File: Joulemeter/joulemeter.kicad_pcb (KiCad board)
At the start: 2 copper layers, 78.9 x 89.7 mm, 50 parts, among them J1 XT60-M, J2 XT60-M, J3 22035035, U2 MCP6286T-E/OT, U5 PADS131M04QPWRQ1

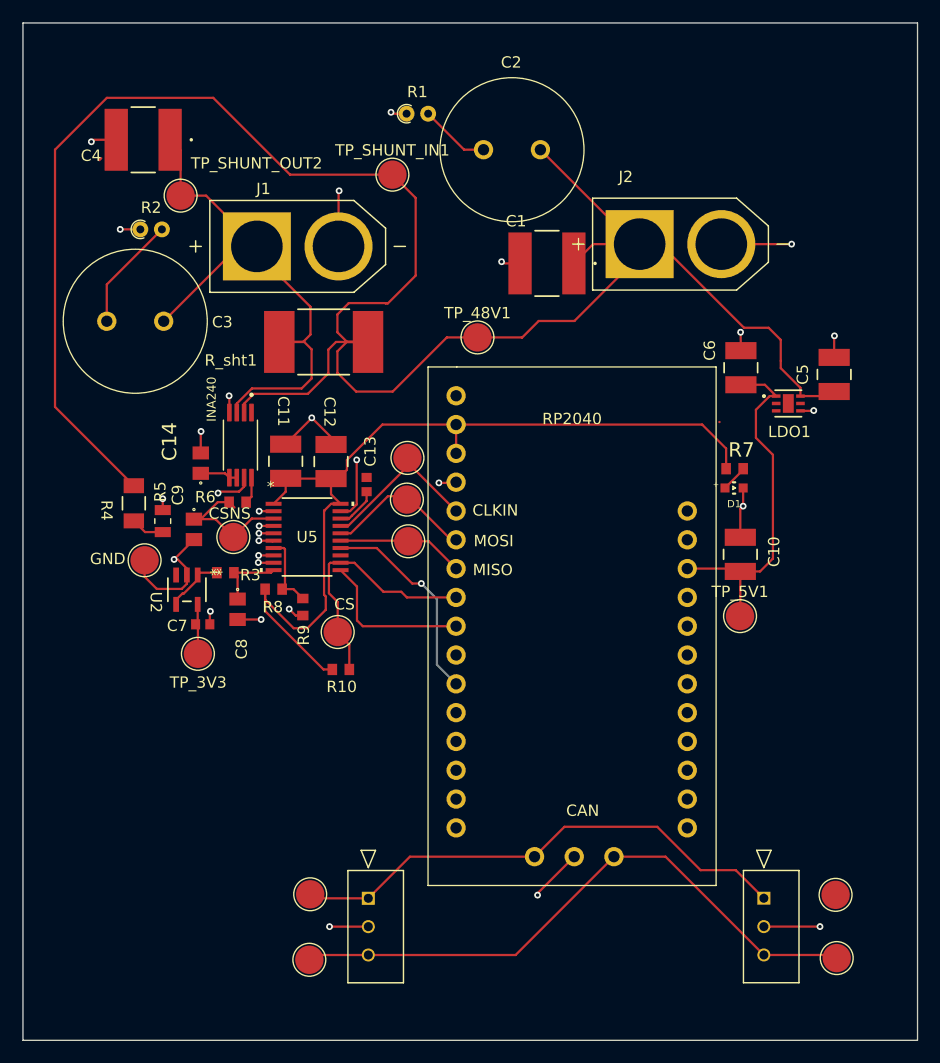
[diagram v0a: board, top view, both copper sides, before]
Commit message: pcb v1384
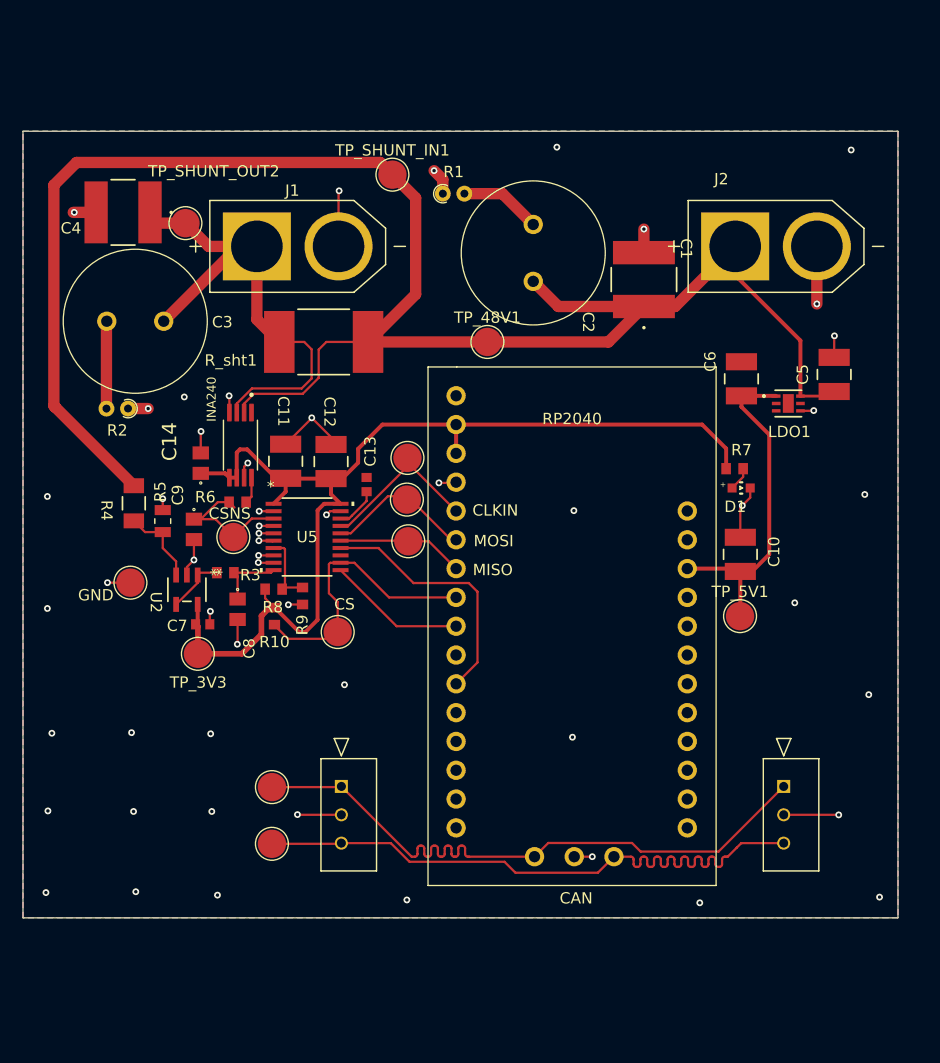
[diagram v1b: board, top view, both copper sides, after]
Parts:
- removed TS_CAN_H2, TS_CAN_L1: ~, TestPoint:TestPoint_Pad_D2.5mm
- moved R2 15.8 mm to (130.2, 89.8), turned to 180 degrees
- moved TS_CAN_L2 10.7 mm to (142.9, 128.2)
- moved J3 10.1 mm to (149.0, 123.2)
- moved TS_CAN_H1 10.0 mm to (142.9, 123.2)
- moved CAN 10.0 mm to (188.0, 123.2)
- moved C2 9.29 mm to (165.9, 76.1), turned to -90 degrees
- moved C1 8.67 mm to (175.7, 78.5), turned to 90 degrees
- moved J2 8.43 mm to (187.3, 75.5)
- moved R1 7.74 mm to (157.9, 70.9)
- moved R10 7.50 mm to (143.1, 108.2), turned to -90 degrees
- moved C4 6.64 mm to (129.8, 72.5)
- moved TP_SHUNT_OUT2 2.46 mm to (135.2, 73.5)
- moved GND 2.34 mm to (130.4, 105.2)
- moved C6 0.98 mm to (184.3, 87.2)
- moved R9 0.97 mm to (145.6, 106.4)
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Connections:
- net /CAN_L renamed CAN_N
- C2 pad 3: (no net) -> +48V
- C2 pad 4: (no net) -> Net-(C2-Pad1)
- CAN pad 1: /CAN_H -> CAN_P
- J3 pad 1: /CAN_H -> CAN_P
- RP2040 pad 31: /CAN_H -> CAN_P
- TS_CAN_H1 pad 1: /CAN_H -> CAN_P
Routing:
- net CAN_P: track 0.00 -> 56.9 mm
- net /CAN_H: track 44.9 -> 0.00 mm
- net +48V: track 197.1 -> 156.1 mm
- net GND: track 85.7 -> 69.9 mm, vias 30 -> 53
- net /SHUNT_LOAD: track 58.4 -> 44.9 mm
- net +3V3: track 88.3 -> 96.1 mm
- net Net-(U2-VIN+): track 2.96 -> 7.23 mm
- net /SCK: track 18.5 -> 22.6 mm, vias 1 -> 0
- net CAN_N: track 53.4 -> 56.7 mm
- net /CS: track 22.6 -> 25.3 mm
- net Net-(C3-Pad1): track 10.1 -> 7.71 mm
- net /RESET: track 14.0 -> 12.2 mm
- net +5V: track 31.7 -> 30.0 mm
- net Net-(C2-Pad1): track 6.20 -> 7.20 mm
- added copper zone on B.Cu, net GND
- added copper zone on F.Cu, net GND
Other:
- board size 78.9 x 89.7 mm -> 77.1 x 69.3 mm
